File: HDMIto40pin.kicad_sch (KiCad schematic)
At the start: 56 parts, among them J17 TTL 40Pin, J18 I2C EDID, U11 LM1117DT-3.3, U12 FAN5333BSX, U13 TFP401APZPR, U14 24LC02BT-E/LT

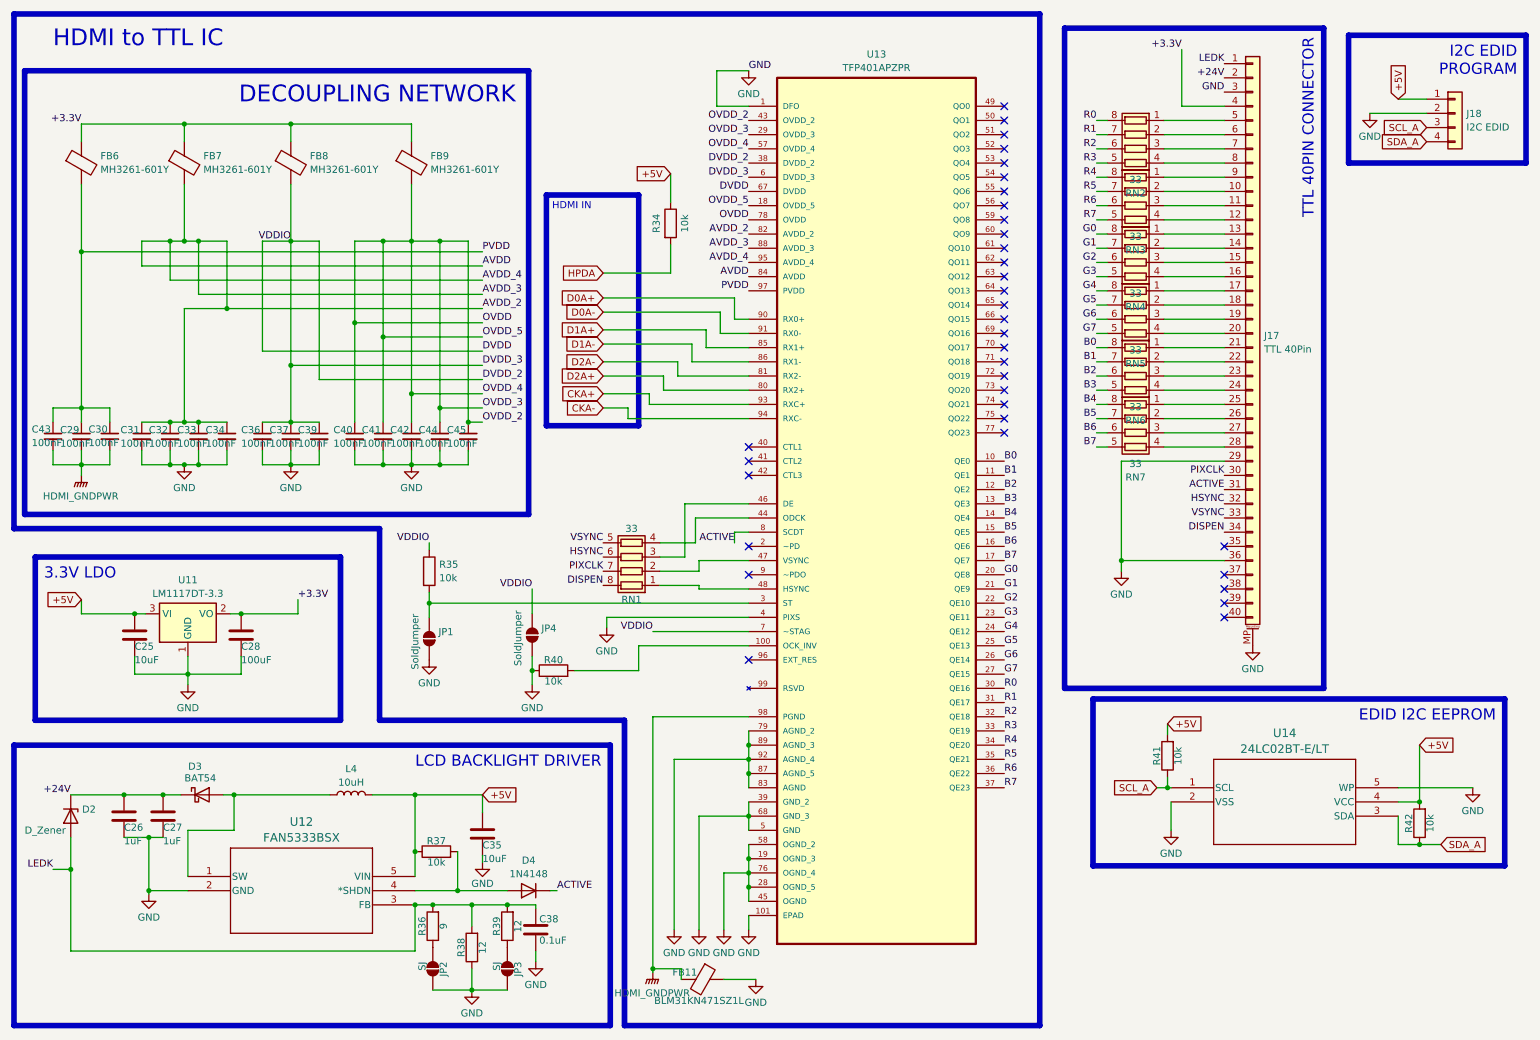
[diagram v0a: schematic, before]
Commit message: update layout pcb & zip tesi
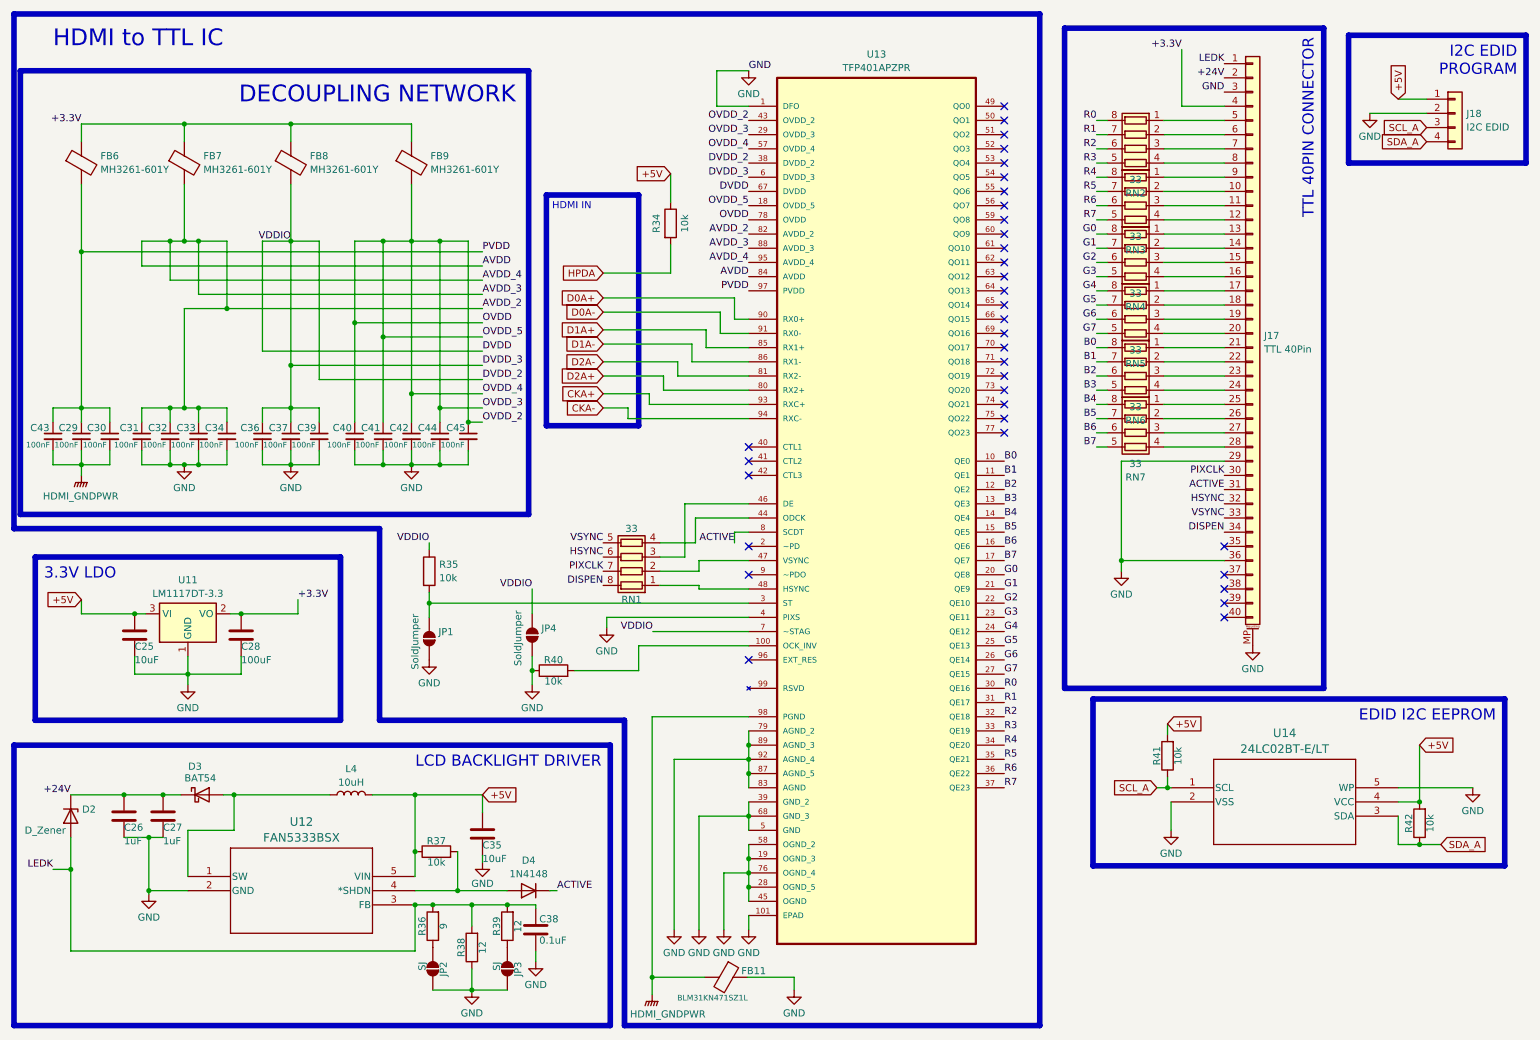
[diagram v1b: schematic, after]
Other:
- moved on the sheet: FB11
